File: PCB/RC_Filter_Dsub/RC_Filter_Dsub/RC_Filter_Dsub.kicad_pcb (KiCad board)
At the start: 2 copper layers, 31.5 x 17.8 mm, 26 parts, among them J1 M83513_13-D01CP, U11 BondPad, U12 BondPad, U13 BondPad, U14 BondPad, U16 BondPad, U17 BondPad, U18 BondPad, U19 BondPad, U2 BondPad, U21 BondPad, U22 BondPad, U23 BondPad, U24 BondPad, U3 BondPad, U4 BondPad, U6 BondPad, U7 BondPad, U8 BondPad, U9 BondPad

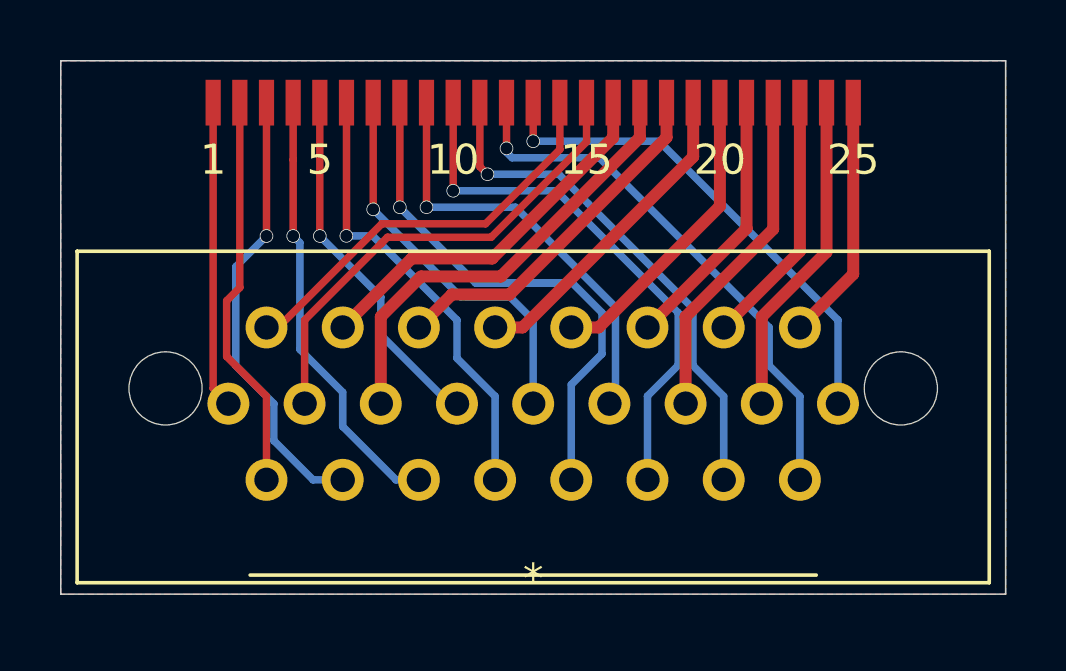
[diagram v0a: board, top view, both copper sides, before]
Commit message: Great
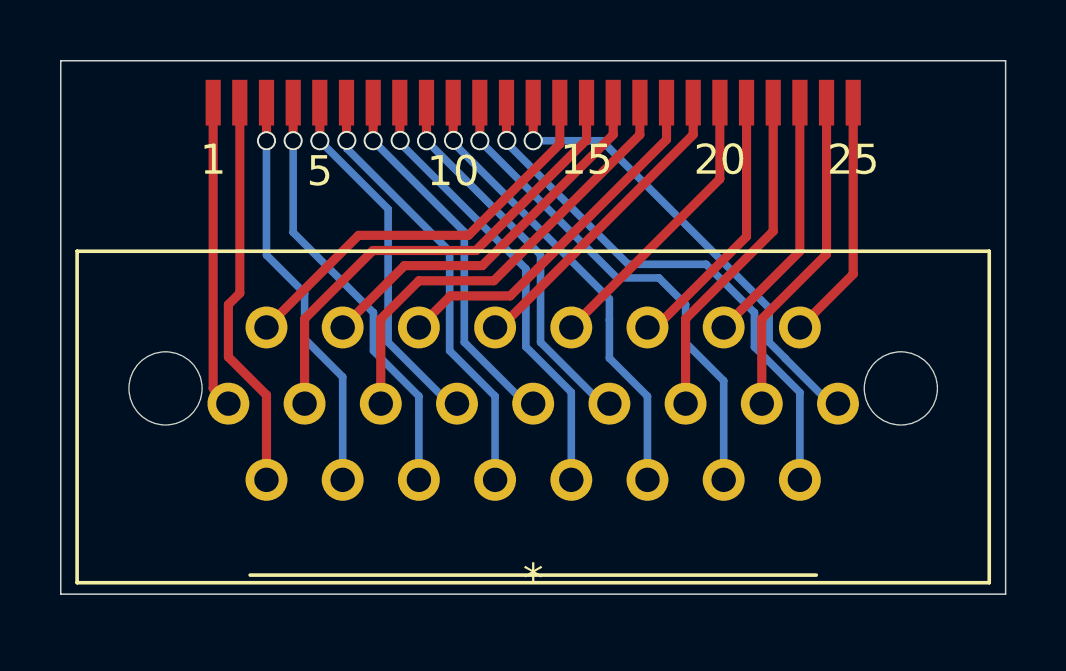
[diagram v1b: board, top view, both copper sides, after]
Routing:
- net Net-(J1-Pad8): track 20.9 -> 14.9 mm
- net Net-(J1-Pad10): track 18.1 -> 15.3 mm
- net Net-(J1-Pad7): track 15.3 -> 13.0 mm
- net Net-(J1-Pad9): track 14.5 -> 13.0 mm
- net Net-(J1-Pad3): track 15.1 -> 13.6 mm
- net Net-(J1-Pad13): track 16.7 -> 15.7 mm
- net Net-(J1-Pad11): track 17.5 -> 16.9 mm
- net Net-(J1-Pad20): track 10.2 -> 9.67 mm
- net Net-(J1-Pad6): track 15.1 -> 14.6 mm
- removed copper zone on B.Cu, net (none)
- removed copper zone on F.Cu, net (none)
